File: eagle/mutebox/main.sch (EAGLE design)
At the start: 33 parts, among them IC1 6N138S-TA1, IC2 6N138S-TA1, IC3 74HCT541DW, IC4 74HCT541DW

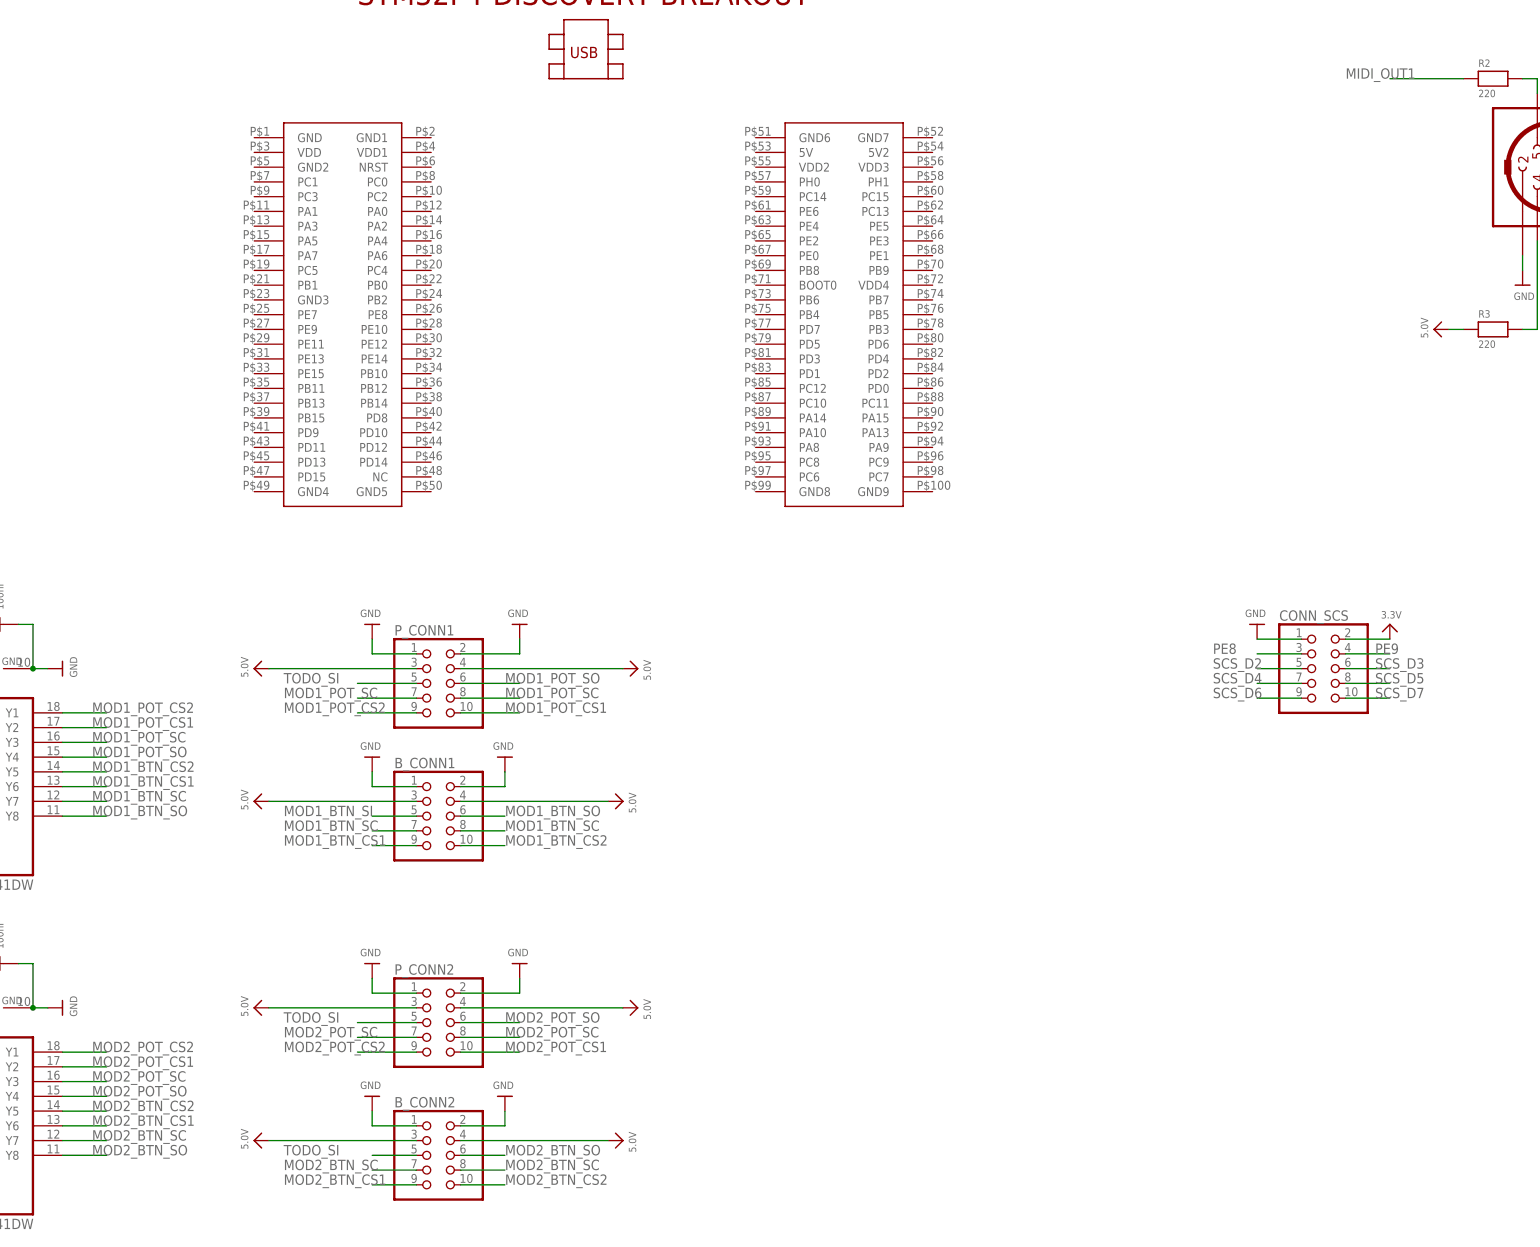
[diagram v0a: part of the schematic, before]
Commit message: muteboxwip
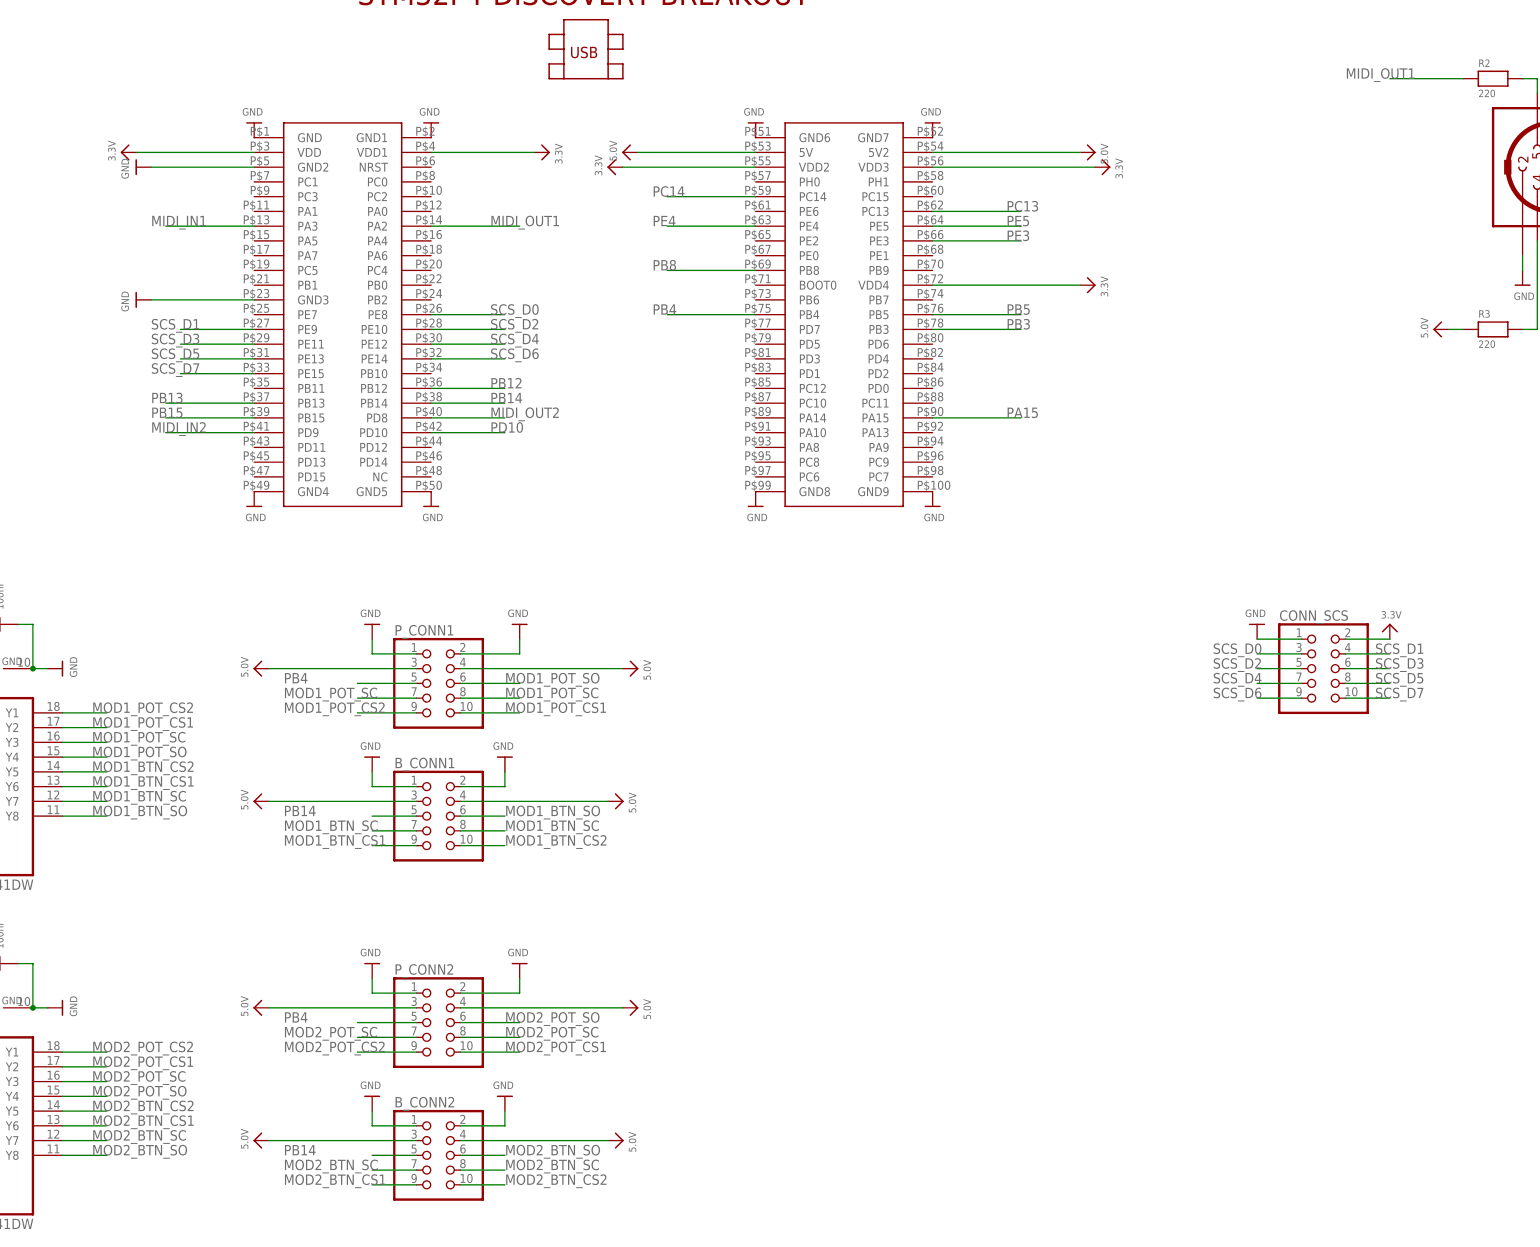
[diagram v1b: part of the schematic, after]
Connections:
- removed net MOD1_BTN_SI: B_CONN1.5
- removed net PE8: CONN_SCS.3
- removed net PE9: CONN_SCS.4
- removed net TODO_SI: B_CONN2.5, P_CONN1.5, P_CONN2.5
- new net PB14: B_CONN1.5, B_CONN2.5, U$1.PB14
- new net PB4: P_CONN1.5, P_CONN2.5, U$1.PB4
- new net PE3: U$1.PE3
- new net SCS_D0: CONN_SCS.3, U$1.PE8
- new net SCS_D1: CONN_SCS.4, U$1.PE9
- net 3.3V: now also U$1.VDD, U$1.VDD1, U$1.VDD2, U$1.VDD3, U$1.VDD4
- net 5.0V: now also U$1.5V, U$1.5V2
- net GND: now also U$1.GND, U$1.GND1, U$1.GND2, U$1.GND3, U$1.GND4, U$1.GND5, U$1.GND6, U$1.GND7, U$1.GND8, U$1.GND9
- net MIDI_IN1: now also U$1.PA3
- net MIDI_IN2: now also U$1.PD9
- net MIDI_OUT1: now also U$1.PA2
- net MIDI_OUT2: now also U$1.PD8
- net PA15: now also U$1.PA15
- net PB12: now also U$1.PB12
- net PB13: now also U$1.PB13
- net PB15: now also U$1.PB15
- net PB3: now also U$1.PB3
- net PB5: now also U$1.PB5
- net PB8: now also U$1.PB8
- net PC13: now also U$1.PC13
- net PC14: now also U$1.PC14
- net PD10: now also U$1.PD10
- net PE4: now also U$1.PE4
- net PE5: now also U$1.PE5
- net SCS_D2: now also U$1.PE10
- net SCS_D3: now also U$1.PE11
- net SCS_D4: now also U$1.PE12
- net SCS_D5: now also U$1.PE13
- net SCS_D6: now also U$1.PE14
- net SCS_D7: now also U$1.PE15
